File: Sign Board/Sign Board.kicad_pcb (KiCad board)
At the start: 2 copper layers, 32 x 68.5 mm, 18 parts, among them J1 Conn_01x03_Socket, J2 Conn_01x03_Pin, J3 Conn_01x03_Pin, J4 Conn_01x03_Pin, J5 Conn_01x03_Pin, J6 Conn_01x03_Pin

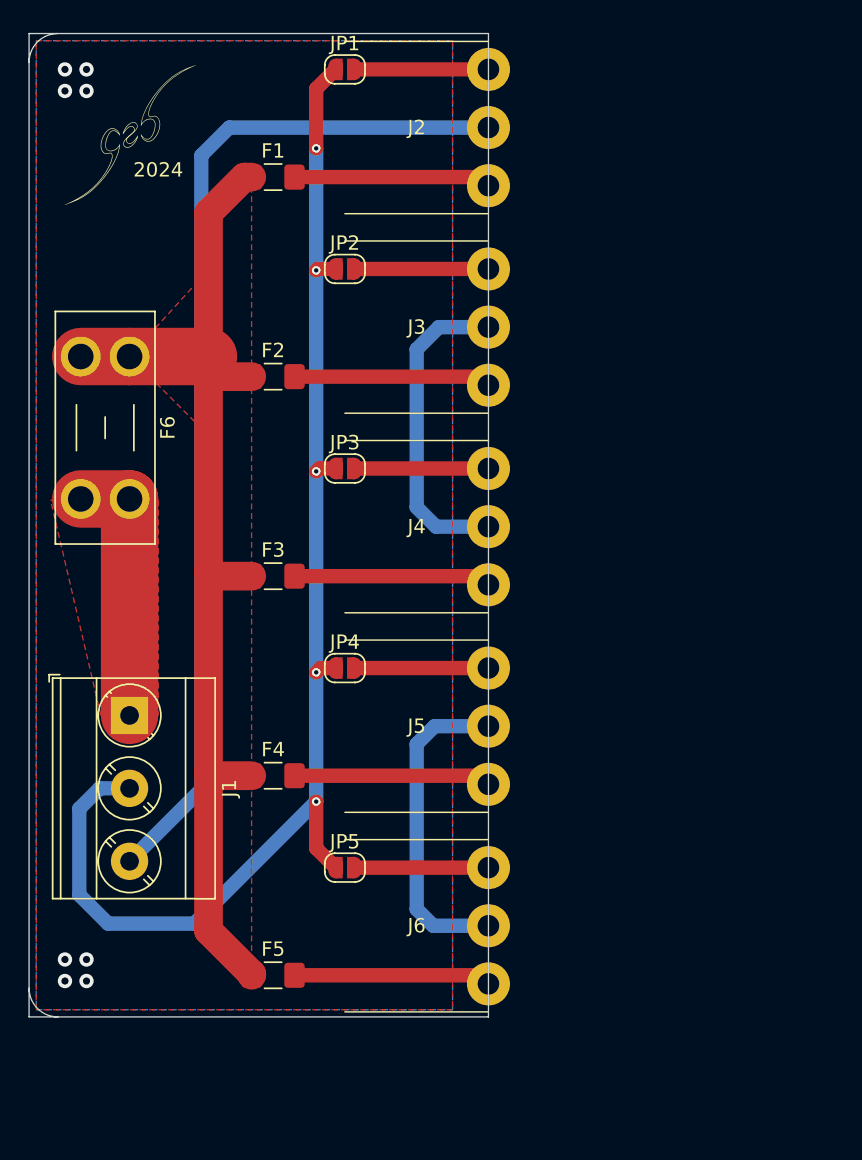
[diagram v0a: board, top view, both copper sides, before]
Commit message: Break Everything
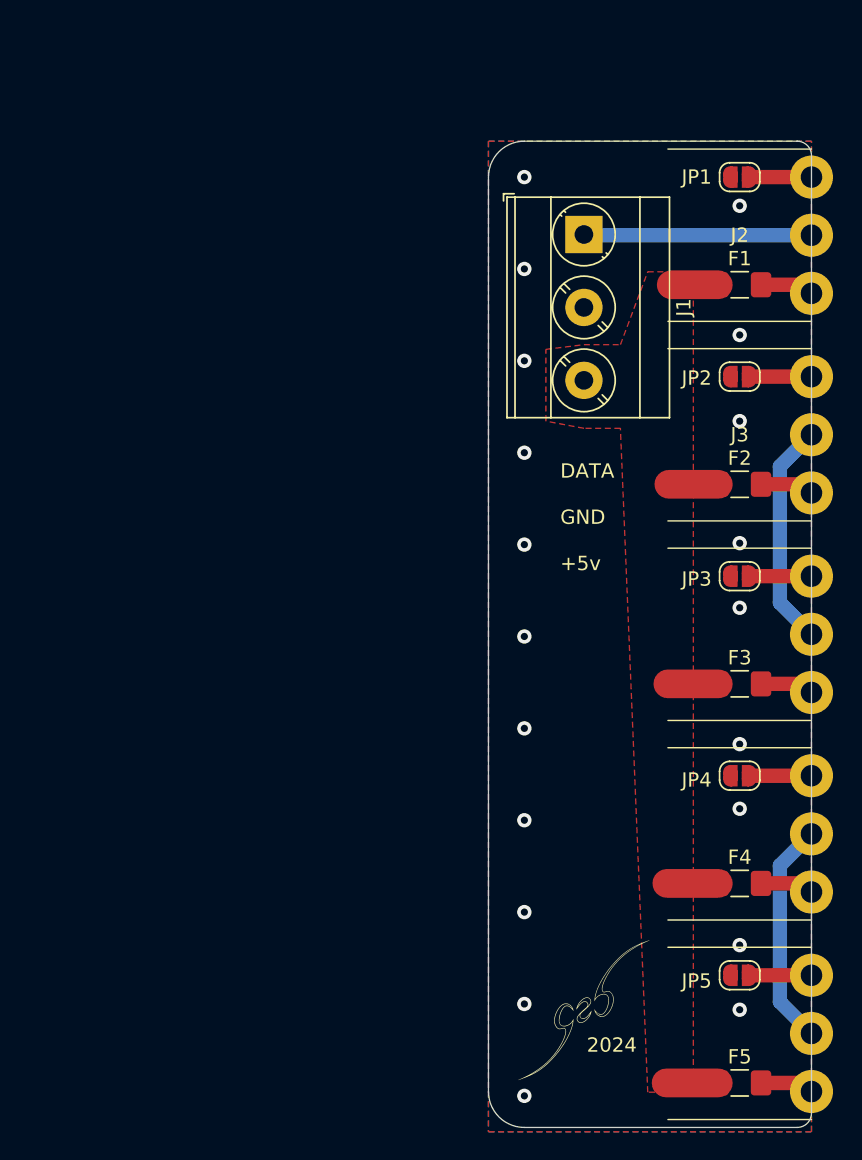
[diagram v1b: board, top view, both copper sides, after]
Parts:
- removed F6: Fuse, Fuse:Fuseholder_Blade_Mini_Keystone_3568
- moved 2024 68.7 mm to (208.6, 123.5)
- moved J1 46.1 mm to (206.7, 66.5)
- moved F1 33.4 mm to (217.5, 70.0)
- moved F2 33.4 mm to (217.5, 83.9)
- moved F3 33.4 mm to (217.5, 97.8)
- moved F4 33.4 mm to (217.5, 111.7)
- moved F5 33.4 mm to (217.5, 125.6)
- moved JP1 28.5 mm to (217.5, 62.5)
- moved JP2 28.5 mm to (217.5, 76.4)
- moved JP3 28.5 mm to (217.5, 90.3)
- moved JP4 28.5 mm to (217.5, 104.2)
- moved JP5 28.5 mm to (217.5, 118.1)
- moved J2 23.7 mm to (222.5, 57.5)
- moved J3 23.7 mm to (222.5, 71.4)
- moved J4 23.7 mm to (222.5, 85.3)
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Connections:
- F1 pad 1: Net-(F1-Pad1) -> Net-(J1-Pin_3)
- F2 pad 1: Net-(F1-Pad1) -> Net-(J1-Pin_3)
- F3 pad 1: Net-(F1-Pad1) -> Net-(J1-Pin_3)
- F4 pad 1: Net-(F1-Pad1) -> Net-(J1-Pin_3)
- F5 pad 1: Net-(F1-Pad1) -> Net-(J1-Pin_3)
- J2 pad 3: Net-(J1-Pin_3) -> Net-(J1-Pin_1)
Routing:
- net Net-(J1-Pin_2): track 92.0 -> 0.00 mm, vias 5 -> 20
- net Net-(F1-Pad1): track 76.6 -> 0.00 mm
- net Net-(J1-Pin_3): track 72.0 -> 17.5 mm
- net Net-(J2-Pin_1): track 13.8 -> 3.76 mm
- net Net-(J6-Pin_1): track 13.8 -> 3.76 mm
- net Net-(J5-Pin_1): track 13.8 -> 3.76 mm
- net Net-(J4-Pin_1): track 13.8 -> 3.76 mm
- net Net-(J3-Pin_1): track 13.8 -> 3.76 mm
- net Net-(J5-Pin_3): track 22.5 -> 15.7 mm
- net Net-(J3-Pin_3): track 22.2 -> 15.7 mm
- net Net-(J6-Pin_2): track 9.35 -> 4.35 mm
- net Net-(J5-Pin_2): track 9.35 -> 4.35 mm
- net Net-(J4-Pin_2): track 8.35 -> 4.35 mm
- net Net-(J3-Pin_2): track 8.35 -> 4.35 mm
- net Net-(J2-Pin_2): track 8.35 -> 4.35 mm
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- added copper zone on F.Cu, net Net-(J1-Pin_3)
- removed copper zone on F.Cu, net Net-(F1-Pad1)
- removed copper zone on F.Cu, net Net-(J1-Pin_1)
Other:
- board size 32 x 68.5 mm -> 22.5 x 68.7 mm
- board text added: "DATA GND +5v"
